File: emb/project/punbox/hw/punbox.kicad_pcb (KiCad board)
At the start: 2 copper layers, 55 x 55 mm, 12 parts, among them J2 Speakers, J3 Button, U1 MAX98357A, U2 MAX98357A

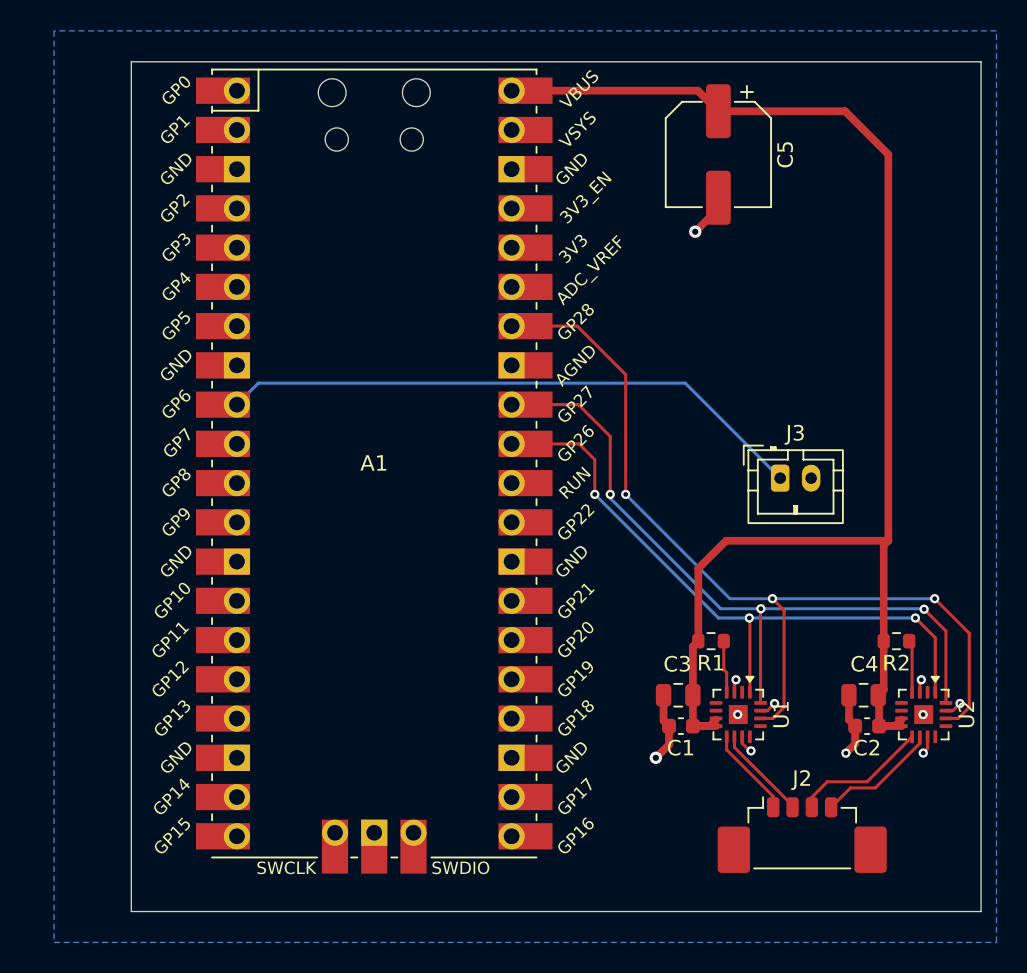
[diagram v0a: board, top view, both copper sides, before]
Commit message: final v1 design
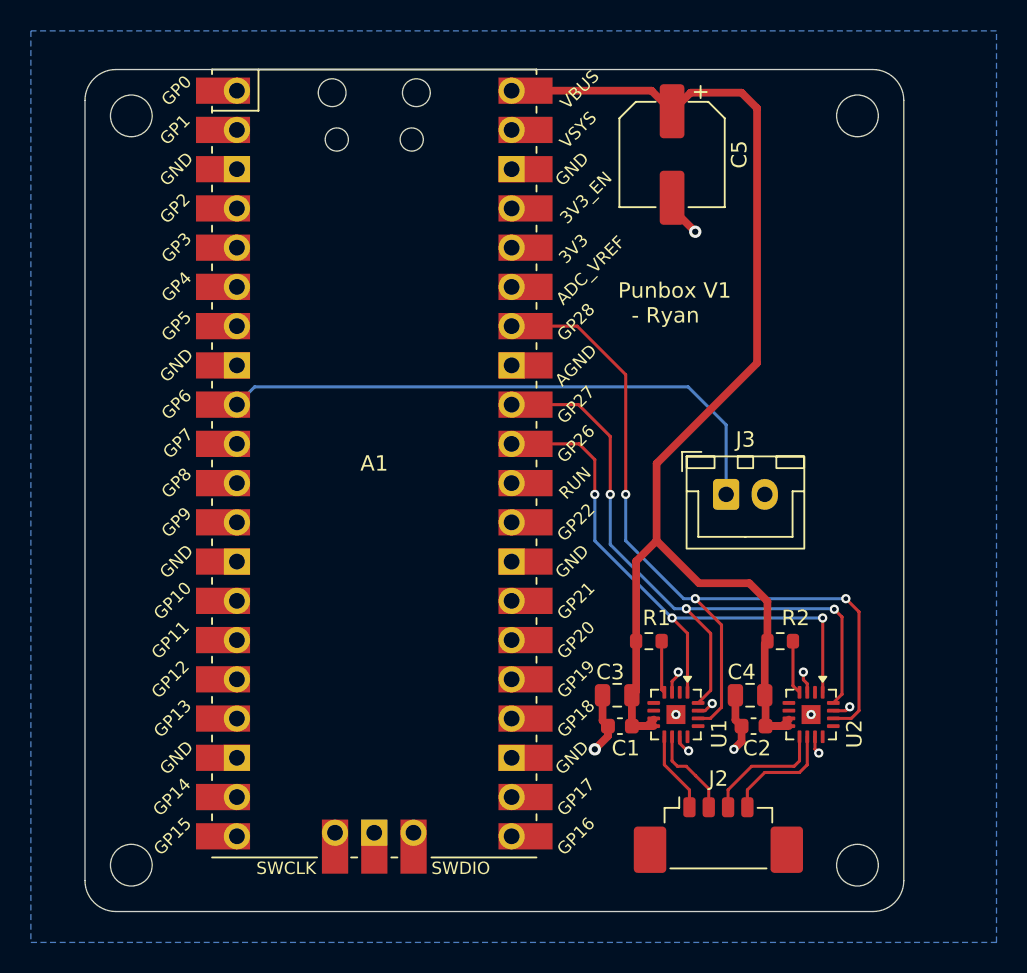
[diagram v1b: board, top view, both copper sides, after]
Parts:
- added REF**: MountingHole_2.7mm_M2.5, MountingHole:MountingHole_2.7mm_M2.5, F.Cu at (127.0, 48.5)
- added REF**: MountingHole_2.7mm_M2.5, MountingHole:MountingHole_2.7mm_M2.5, F.Cu at (127.0, 97.0)
- added REF**: MountingHole_2.7mm_M2.5, MountingHole:MountingHole_2.7mm_M2.5, F.Cu at (80.0, 97.0)
- added REF**: MountingHole_2.7mm_M2.5, MountingHole:MountingHole_2.7mm_M2.5, F.Cu at (80.0, 48.5)
- J3: footprint punbox_parts:JST_PH_B2B-PH-K_1x02_P2.00mm_Vertical -> punbox_parts:JST_XH_B2B-XH-A_1x02_P2.50mm_Vertical
- moved R2 7.53 mm to (122.0, 82.5)
- moved C4 7.35 mm to (120.0, 86.0)
- moved C2 7.35 mm to (120.3, 88.0)
- moved U2 7.29 mm to (124.0, 87.2)
- moved J2 5.42 mm to (118.0, 94.5)
- moved U1 4.04 mm to (115.2, 87.2)
- moved R1 4.03 mm to (113.5, 82.5)
- moved C1 3.95 mm to (111.6, 88.0)
- moved C3 3.95 mm to (111.5, 86.0)
- moved J3 3.65 mm to (118.5, 73.0)
- moved C5 3.00 mm to (115.0, 51.0)
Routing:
- net +5V: track 93.0 -> 83.9 mm
- net I2S_DIN: track 42.3 -> 37.9 mm
- net I2S_LRCLK: track 58.2 -> 54.3 mm
- net I2S_BCLK: track 47.5 -> 44.2 mm
- net N$3: track 8.76 -> 8.09 mm
- net BUTTON: track 38.3 -> 37.7 mm
- net N$1: track 5.81 -> 5.24 mm
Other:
- board size 55 x 55 mm -> 53 x 54.5 mm
- board text added: "Punbox V1 - Ryan"
